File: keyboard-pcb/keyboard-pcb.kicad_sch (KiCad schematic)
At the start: 131 parts

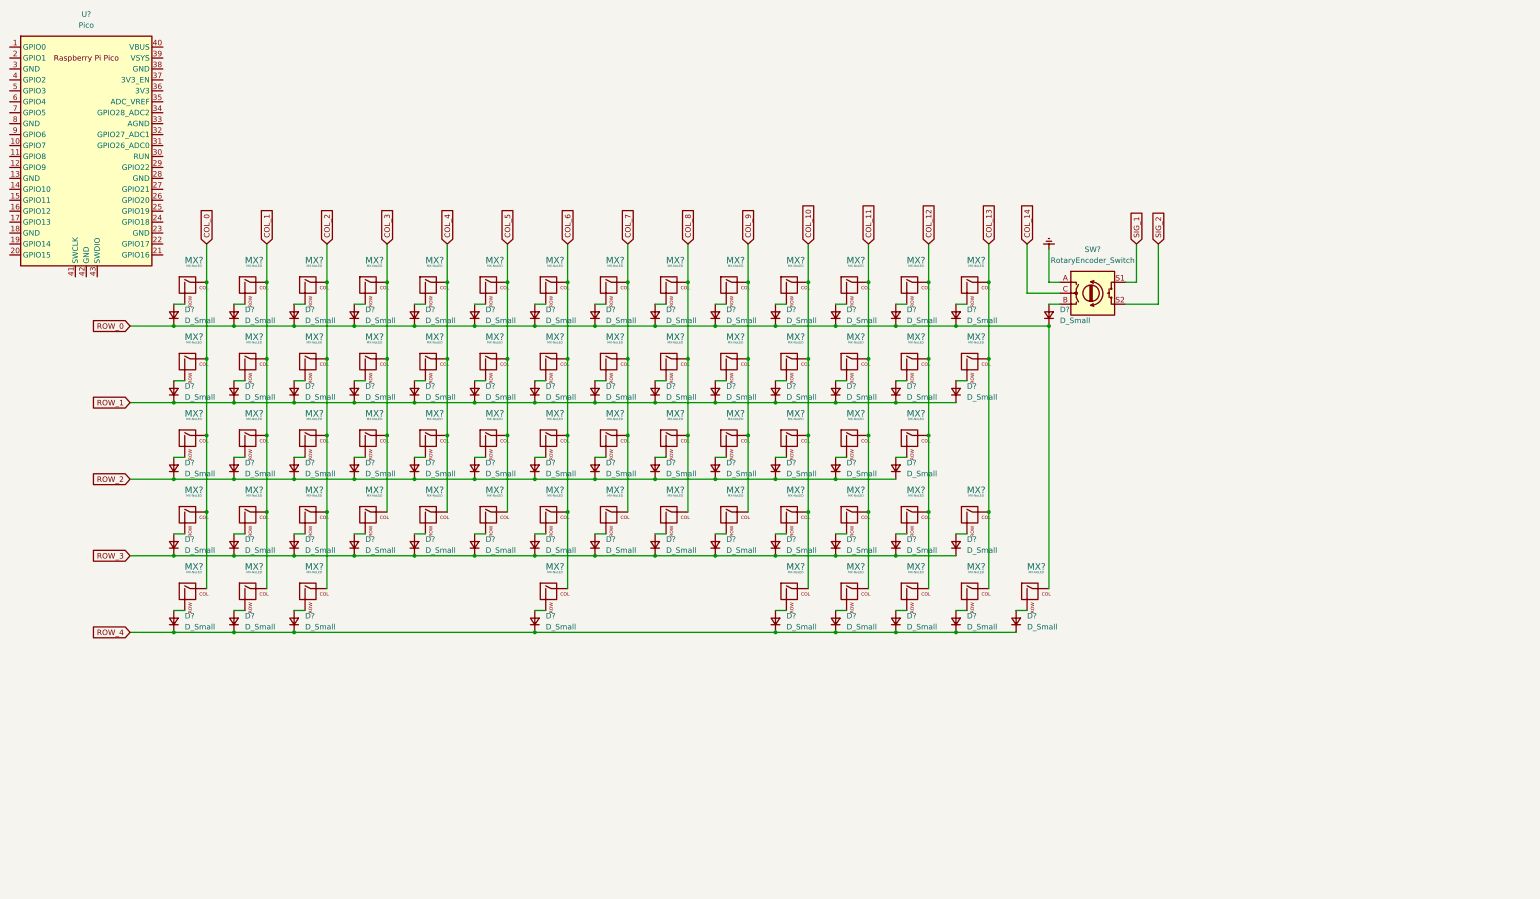
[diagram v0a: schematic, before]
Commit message: labelling rows/columns/connections in schematic
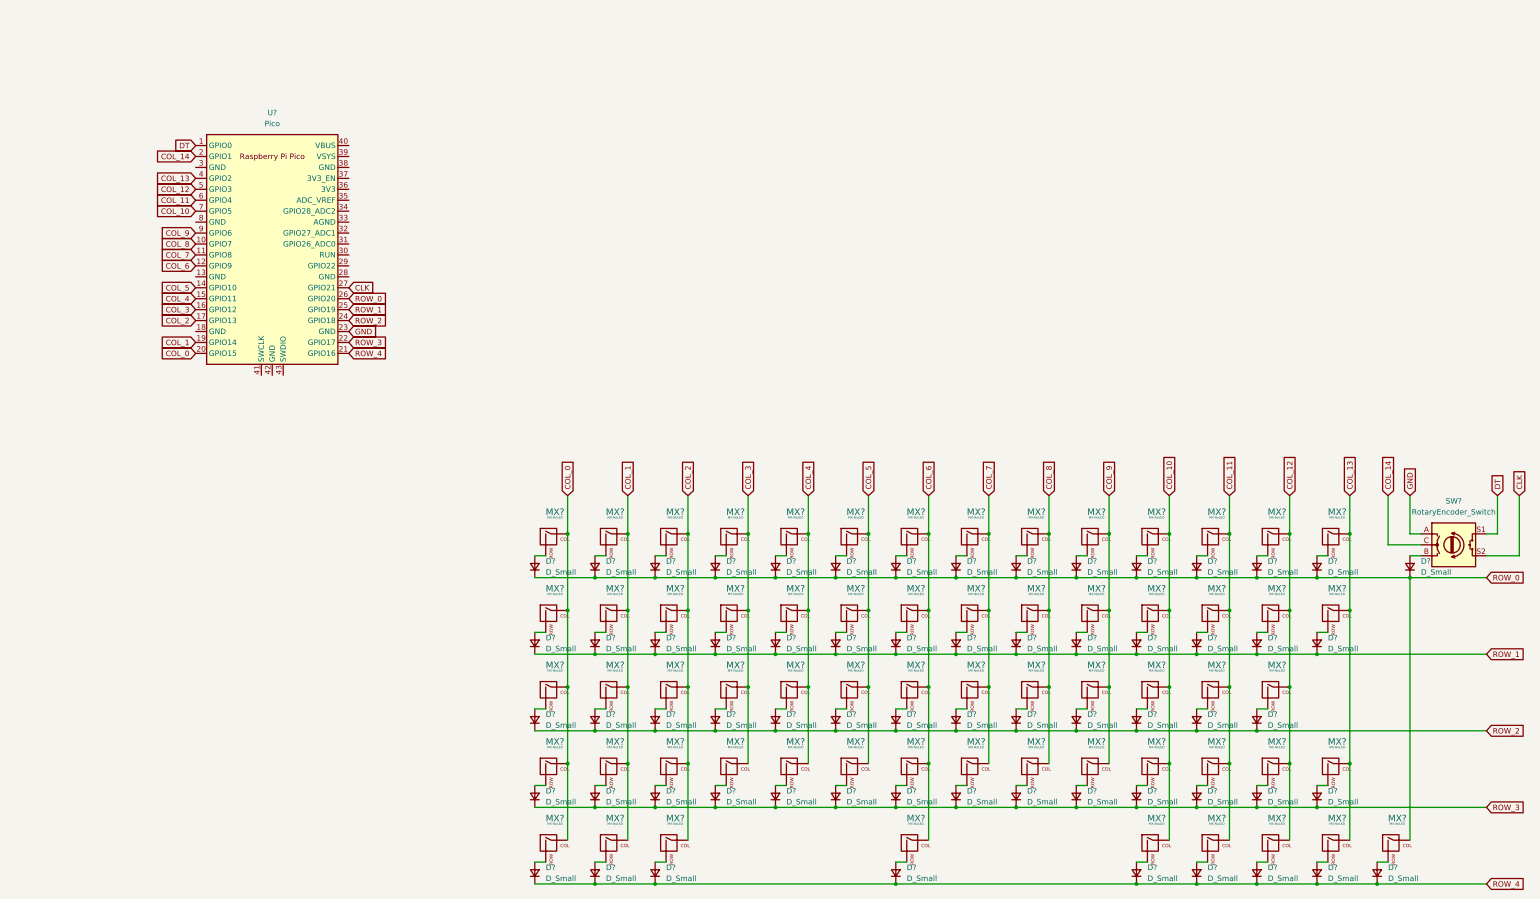
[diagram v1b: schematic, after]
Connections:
- net Earth is gone; now on net GND: SW?.A
- net SIG_1 is gone; now on net DT: SW?.S1
- net SIG_2 is gone; now on net CLK: SW?.S2
- net COL_0: now also U?.20 (GPIO15)
- net COL_1: now also U?.19 (GPIO14)
- net COL_10: now also U?.7 (GPIO5)
- net COL_11: now also U?.6 (GPIO4)
- net COL_12: now also U?.5 (GPIO3)
- net COL_13: now also U?.4 (GPIO2)
- net COL_14: now also U?.2 (GPIO1)
- net COL_2: now also U?.17 (GPIO13)
- net COL_3: now also U?.16 (GPIO12)
- net COL_4: now also U?.15 (GPIO11)
- net COL_5: now also U?.14 (GPIO10)
- net COL_6: now also U?.12 (GPIO9)
- net COL_7: now also U?.11 (GPIO8)
- net COL_8: now also U?.10 (GPIO7)
- net COL_9: now also U?.9 (GPIO6)
- net ROW_0: now also U?.26 (GPIO20)
- net ROW_1: now also U?.25 (GPIO19)
- net ROW_2: now also U?.24 (GPIO18)
- net ROW_3: now also U?.22 (GPIO17)
- net ROW_4: now also U?.21 (GPIO16)
- net DT: now reaches U?.1 (GPIO0)
- net GND: now reaches U?.23 (GND)
- net CLK: now reaches U?.27 (GPIO21)
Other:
- moved on the sheet: D?, MX?, SW?, U?

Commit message: removed column from schematic
- making it more efficient use of GPIO pins
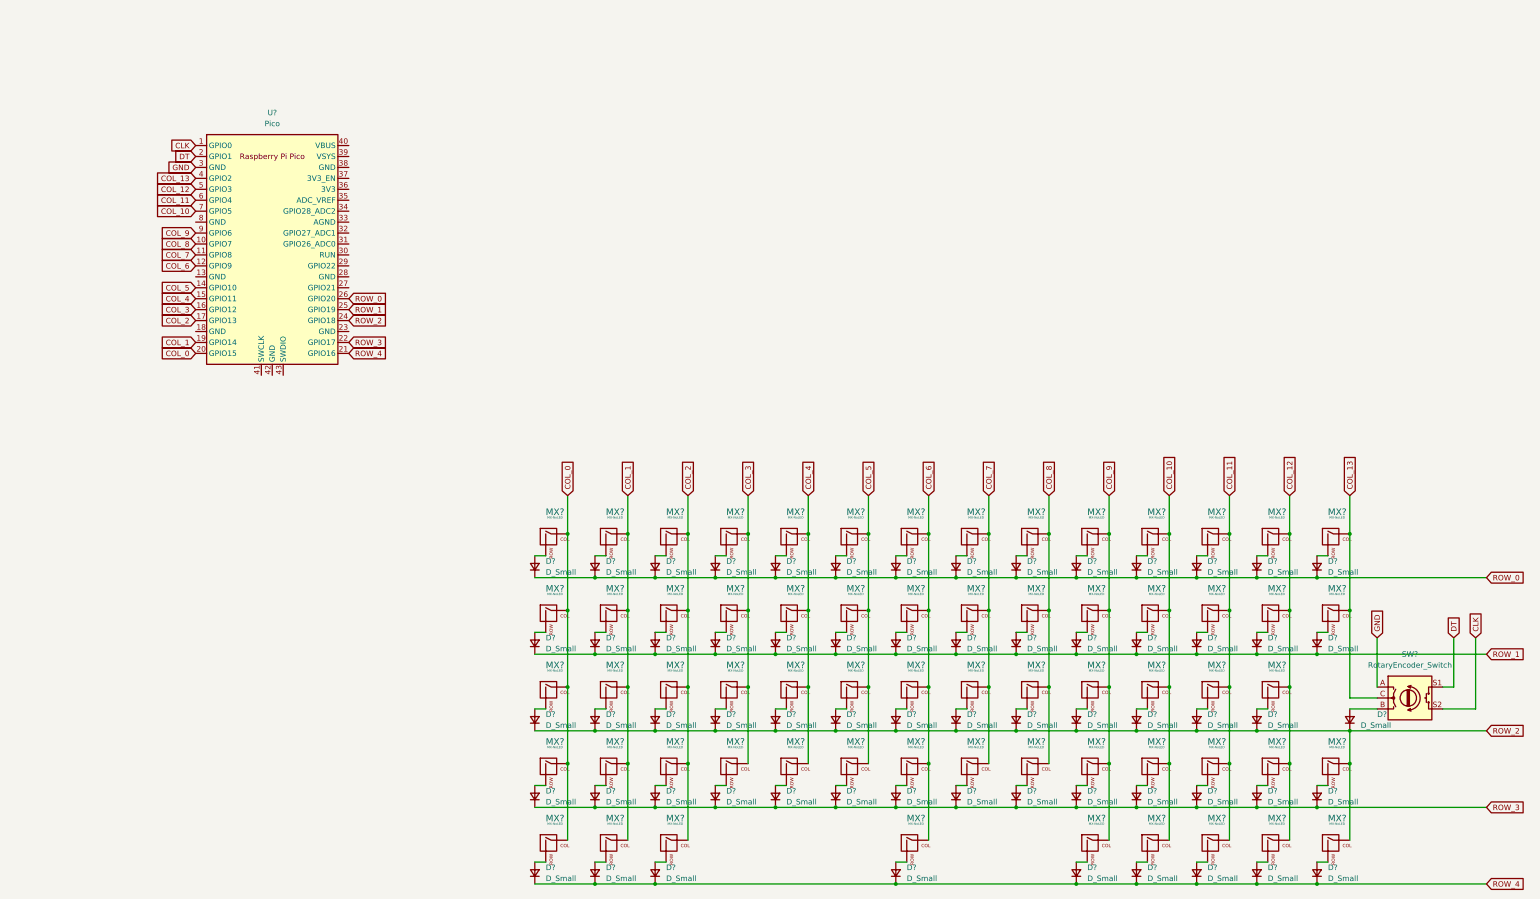
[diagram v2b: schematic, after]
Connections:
- net CLK: now also U?.1 (GPIO0); no longer U?.27 (GPIO21)
- net COL_10: now also MX?.1 (COL); no longer MX?.1 (COL)
- net COL_11: now also MX?.1 (COL); no longer MX?.1 (COL)
- net COL_12: now also MX?.1 (COL); no longer MX?.1 (COL)
- net COL_13: now also SW?.C; no longer MX?.1 (COL), MX?.1 (COL)
- net COL_9: now also MX?.1 (COL)
- net DT: now also U?.2 (GPIO1); no longer U?.1 (GPIO0)
- net GND: now also U?.3 (GND); no longer U?.23 (GND)
- net ROW_0: no longer D?.1 (K), MX?.1 (COL)
- net ROW_2: now also D?.1 (K), MX?.1 (COL), MX?.1 (COL)
- removed net COL_14: SW?.C, U?.2 (GPIO1)
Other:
- moved on the sheet: D?, MX?, SW?

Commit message: Revert "removed column from schematic"
This reverts commit 2b4230f3693d24e53e3d9f57aeab1cc1c25adc82.
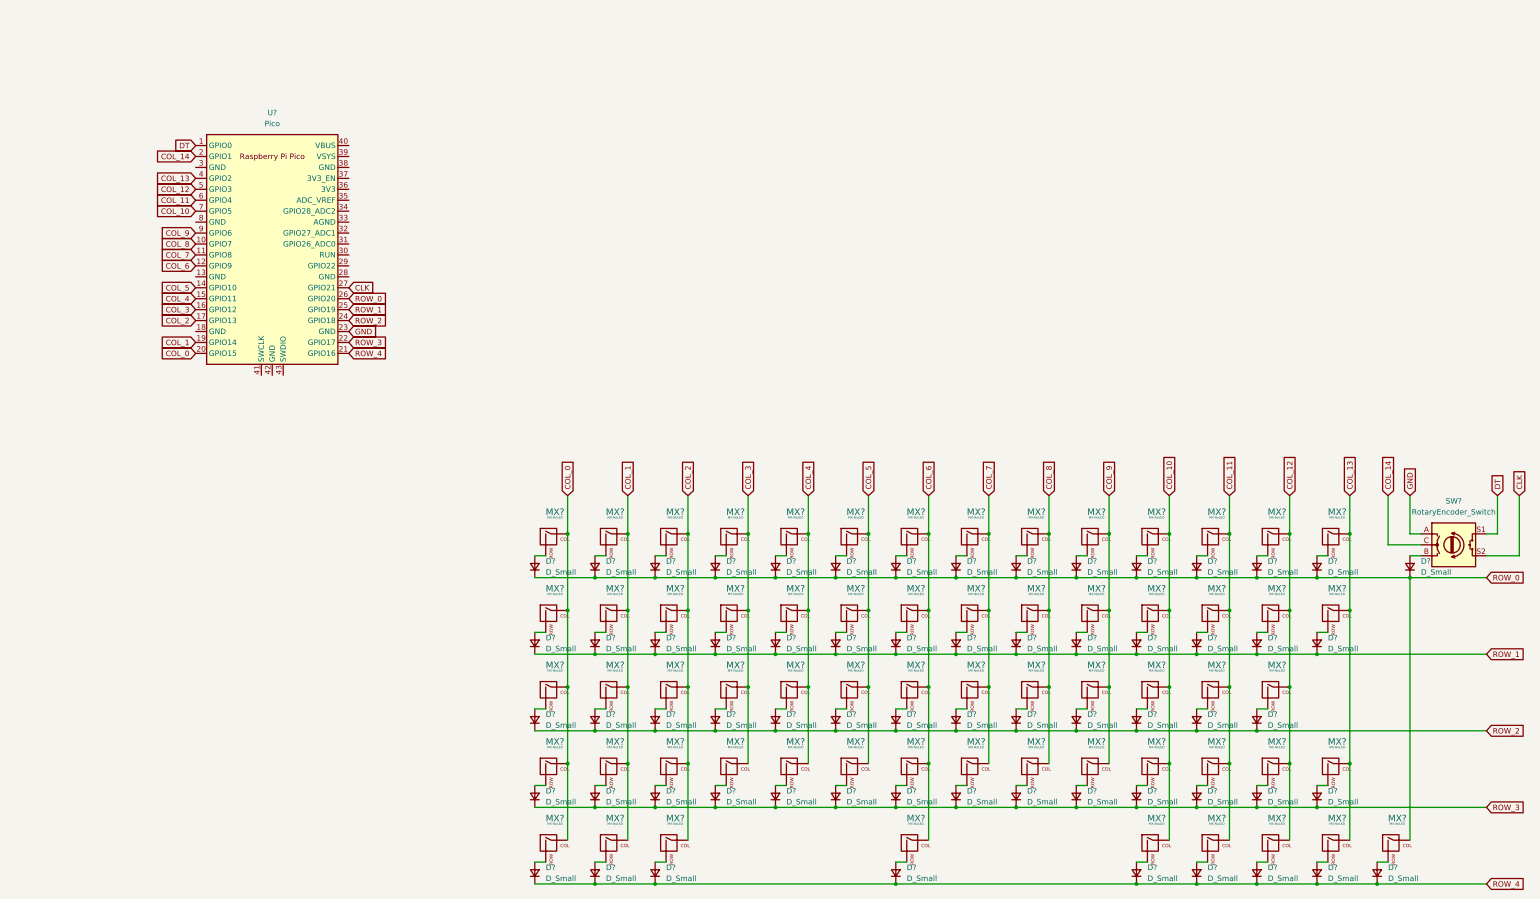
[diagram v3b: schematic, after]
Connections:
- net CLK: now also U?.27 (GPIO21); no longer U?.1 (GPIO0)
- net COL_10: now also MX?.1 (COL); no longer MX?.1 (COL)
- net COL_11: now also MX?.1 (COL); no longer MX?.1 (COL)
- net COL_12: now also MX?.1 (COL); no longer MX?.1 (COL)
- net COL_13: now also MX?.1 (COL), MX?.1 (COL); no longer SW?.C
- net COL_9: no longer MX?.1 (COL)
- net DT: now also U?.1 (GPIO0); no longer U?.2 (GPIO1)
- net GND: now also U?.23 (GND); no longer U?.3 (GND)
- net ROW_0: now also D?.1 (K), MX?.1 (COL)
- net ROW_2: no longer D?.1 (K), MX?.1 (COL), MX?.1 (COL)
- new net COL_14: SW?.C, U?.2 (GPIO1)
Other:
- moved on the sheet: D?, MX?, SW?
